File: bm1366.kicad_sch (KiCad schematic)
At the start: 7 parts, among them J2 Conn_01x06, U35 TXU0304PW, U8 25MHz

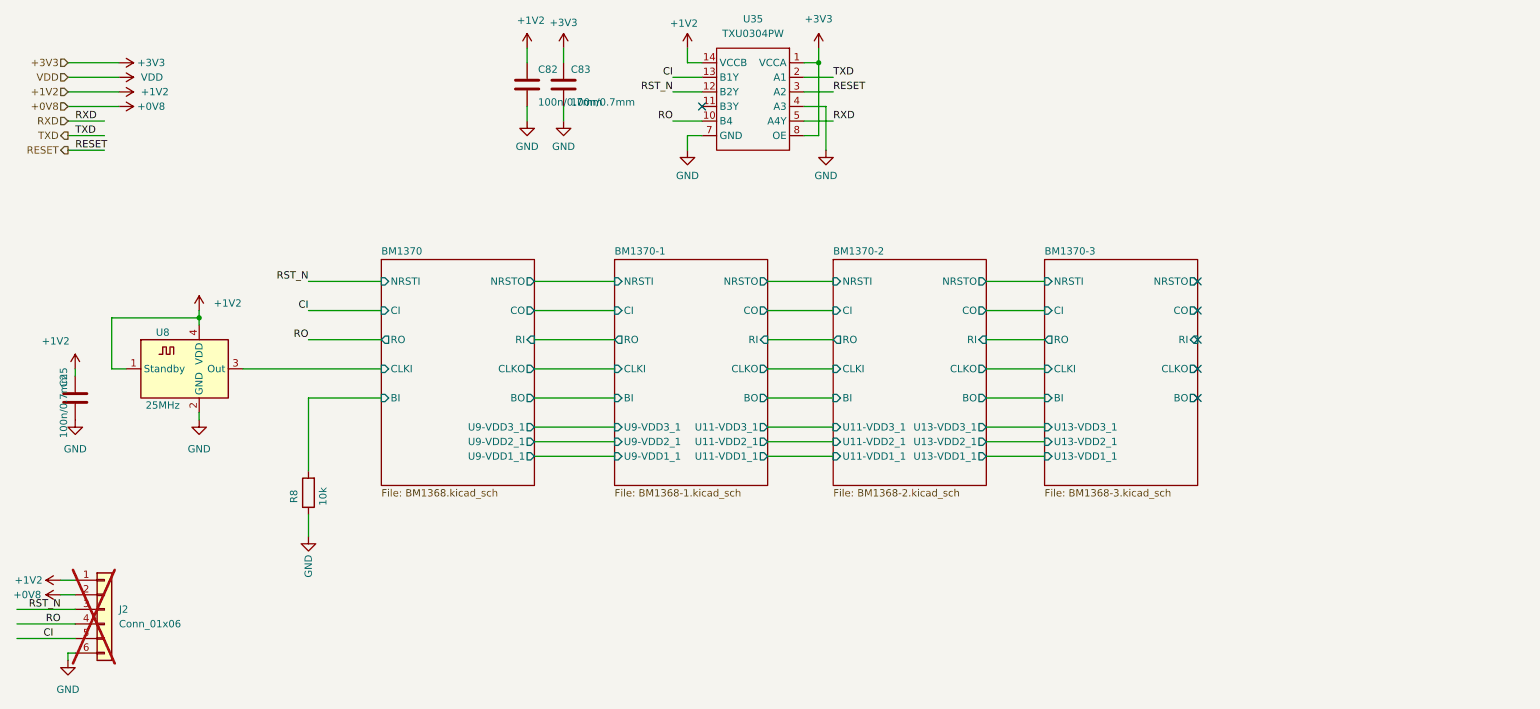
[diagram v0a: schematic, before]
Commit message: 0502
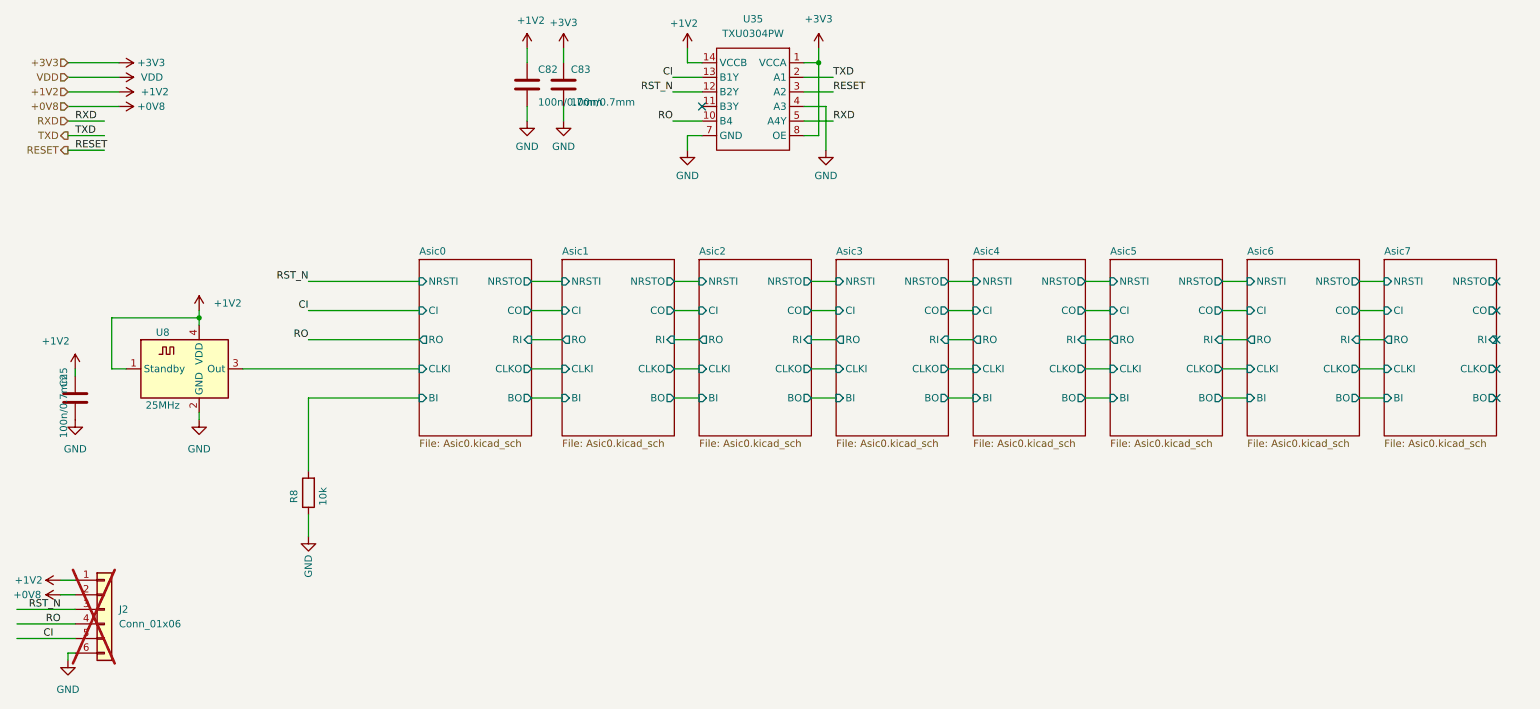
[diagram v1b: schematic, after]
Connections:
- net BM1370/BI renamed Asic0/BI
- net BM1370/CLKI renamed Asic0/CLKI
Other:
- removed sheet BM1370
- removed sheet BM1370-1
- removed sheet BM1370-2
- removed sheet BM1370-3
- added sheet Asic0 (Asic0.kicad_sch)
- added sheet Asic1 (Asic0.kicad_sch)
- added sheet Asic2 (Asic0.kicad_sch)
- added sheet Asic3 (Asic0.kicad_sch)
- added sheet Asic4 (Asic0.kicad_sch)
- added sheet Asic5 (Asic0.kicad_sch)
- added sheet Asic6 (Asic0.kicad_sch)
- added sheet Asic7 (Asic0.kicad_sch)
